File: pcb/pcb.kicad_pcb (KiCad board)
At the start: 2 copper layers, 1 part

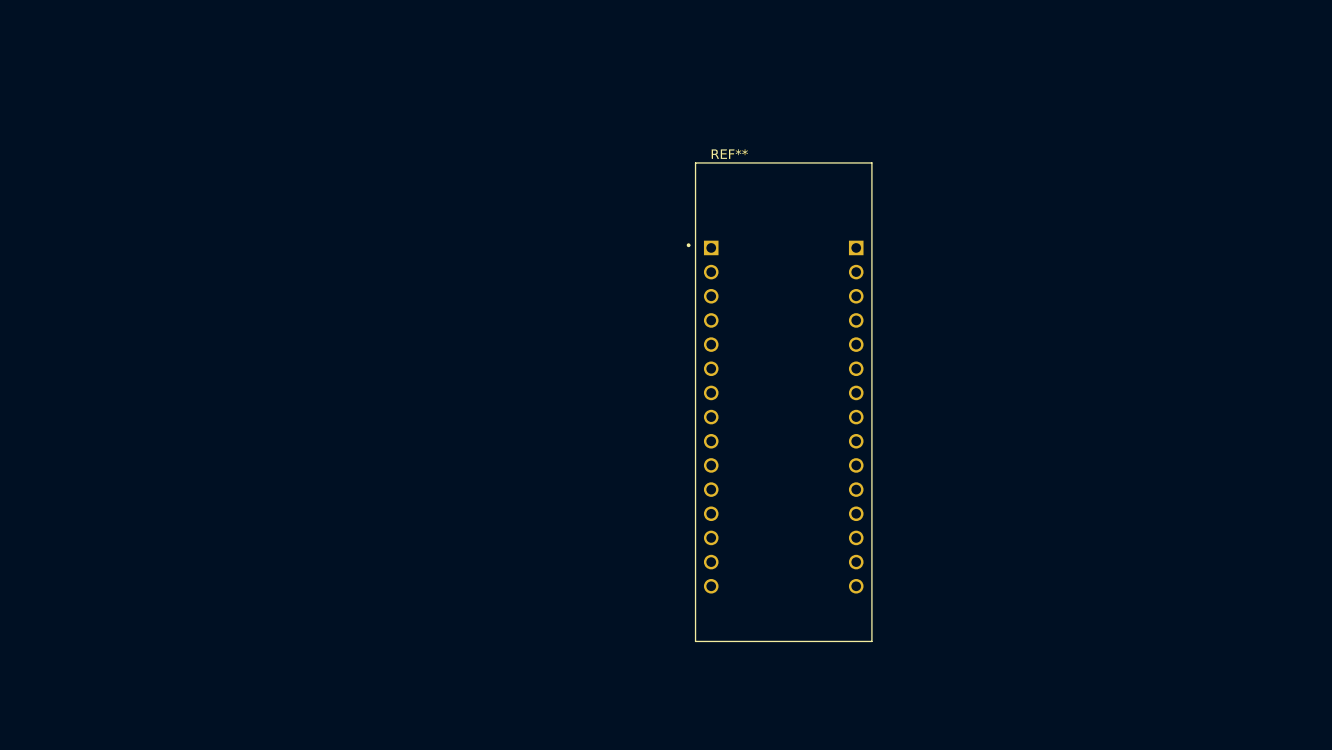
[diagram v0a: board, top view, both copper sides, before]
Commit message: Finalisation PCB
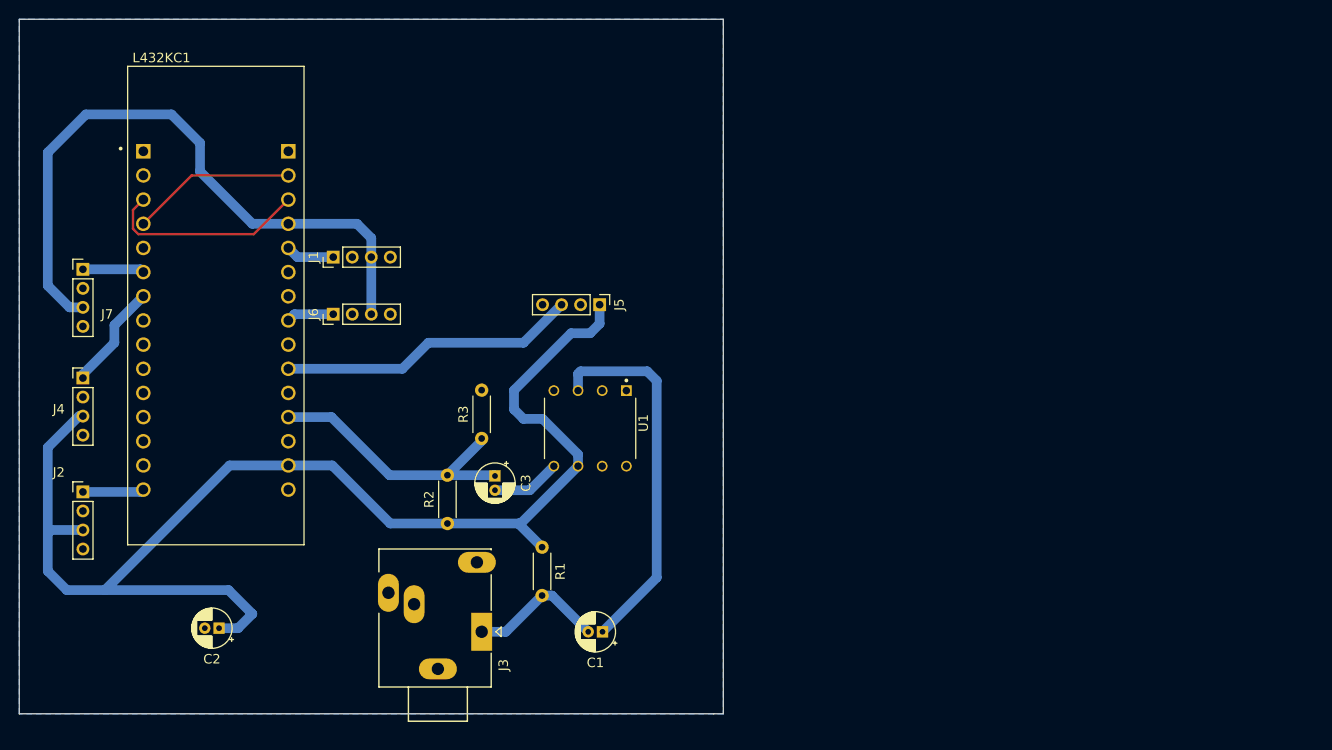
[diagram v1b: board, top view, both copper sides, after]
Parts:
- removed REF**: MODULE_NUCLEO-L432KC, NUCLEO-L432KC:MODULE_NUCLEO-L432KC
- added C1: 1n, Capacitor_THT:CP_Radial_D4.0mm_P1.50mm, F.Cu at (114.3, 119.4)
- added C2: 10u, Capacitor_THT:CP_Radial_D4.0mm_P1.50mm, F.Cu at (74.0, 119.0)
- added C3: 1u, Capacitor_THT:CP_Radial_D4.0mm_P1.50mm, F.Cu at (103.0, 103.0)
- added J1: VIN VBAT, Connector_PinHeader_2.00mm:PinHeader_1x04_P2.00mm_Vertical, F.Cu at (86.0, 80.0)
- added J2: Conn_01x04, Connector_PinHeader_2.00mm:PinHeader_1x04_P2.00mm_Vertical, F.Cu at (59.7, 104.7)
- added J3: AudioJack3, Connector_Audio:Jack_3.5mm_Ledino_KB3SPRS_Horizontal, F.Cu at (101.6, 119.4)
- added J4: Conn_01x04, Connector_PinHeader_2.00mm:PinHeader_1x04_P2.00mm_Vertical, F.Cu at (59.7, 92.7)
- added J5: HX711, Connector_PinHeader_2.00mm:PinHeader_1x04_P2.00mm_Vertical, F.Cu at (114.0, 85.0)
- added J6: Conn_01x04, Connector_PinHeader_2.00mm:PinHeader_1x04_P2.00mm_Vertical, F.Cu at (86.0, 86.0)
- added J7: Conn_01x04, Connector_PinHeader_2.00mm:PinHeader_1x04_P2.00mm_Vertical, F.Cu at (59.7, 81.3)
- added L432KC1: NUCLEO_L432KC, NUCLEO-L432KC:MODULE_NUCLEO-L432KC, F.Cu at (73.7, 85.1)
- added R1: 4.7k, Resistor_THT:R_Axial_DIN0204_L3.6mm_D1.6mm_P5.08mm_Horizontal, F.Cu at (108.0, 110.5)
- added R2: 10k, Resistor_THT:R_Axial_DIN0204_L3.6mm_D1.6mm_P5.08mm_Horizontal, F.Cu at (98.0, 108.0)
- added R3: 10k, Resistor_THT:R_Axial_DIN0204_L3.6mm_D1.6mm_P5.08mm_Horizontal, F.Cu at (101.6, 99.1)
- added U1: LM386, LM386N-4_NOPB:DIP794W45P254L959H508Q8, F.Cu at (113.0, 98.0)
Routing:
- net /+3V3: track 0.00 -> 138.9 mm
- net /+5V: track 0.00 -> 69.4 mm
- net Net-(C1-Pad1): track 0.00 -> 39.3 mm
- net /A2: track 0.00 -> 31.5 mm
- net /A0: track 0.00 -> 29.6 mm
- net Net-(L432KC1-PadNRST): track 0.00 -> 21.6 mm
- net GND: track 0.00 -> 17.3 mm
- net Net-(C1-Pad2): track 0.00 -> 14.4 mm
- net /D4: track 0.00 -> 11.2 mm
- net Net-(C3-Pad2): track 0.00 -> 7.24 mm
- net /D3: track 0.00 -> 6.47 mm
- net /D12: track 0.00 -> 6.45 mm
- net /A7: track 0.00 -> 5.12 mm
- net /A4: track 0.00 -> 4.99 mm
- added copper zone on B.Cu, net GND
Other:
- board outline added: 74 x 73 mm
- board text added: "HX711"

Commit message: Finalisation PCB
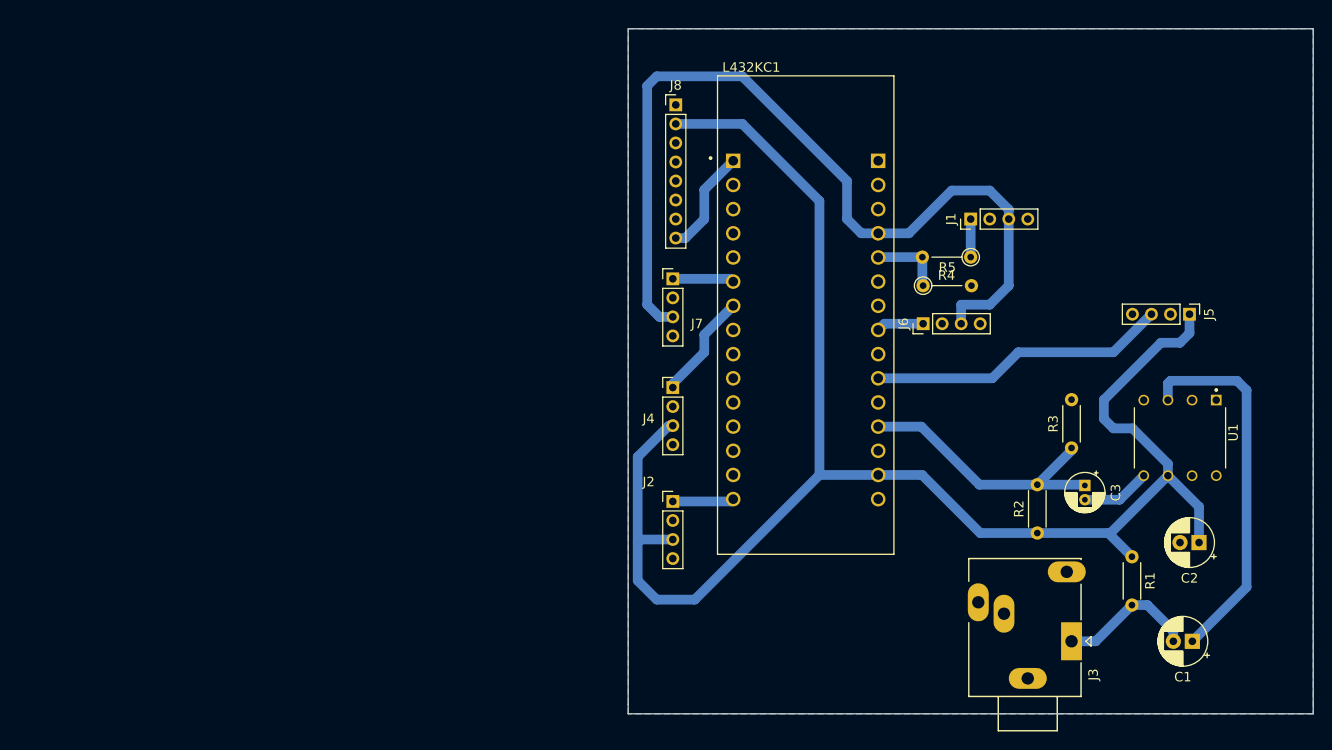
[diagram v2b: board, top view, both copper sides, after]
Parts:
- added J8: Conn_01x08, Connector_PinHeader_2.00mm:PinHeader_1x08_P2.00mm_Vertical, F.Cu at (122.0, 64.0)
- added R4: 2k, Resistor_THT:R_Axial_DIN0204_L3.6mm_D1.6mm_P5.08mm_Vertical, F.Cu at (153.0, 80.0)
- added R5: 1k, Resistor_THT:R_Axial_DIN0204_L3.6mm_D1.6mm_P5.08mm_Vertical, F.Cu at (148.0, 83.0)
- C1: value 1n -> 1u; footprint Capacitor_THT:CP_Radial_D4.0mm_P1.50mm -> Capacitor_THT:CP_Radial_D5.0mm_P2.00mm
- C2: footprint Capacitor_THT:CP_Radial_D4.0mm_P1.50mm -> Capacitor_THT:CP_Radial_D5.0mm_P2.00mm
- moved C2 103.4 mm to (177.0, 110.0)
- moved J1 67.1 mm to (153.0, 76.0)
- moved C1 62.0 mm to (176.3, 120.4)
- moved C3 62.0 mm to (165.0, 104.0)
- moved J2 62.0 mm to (121.7, 105.7)
- moved J3 62.0 mm to (163.6, 120.4)
- moved J4 62.0 mm to (121.7, 93.7)
- moved J5 62.0 mm to (176.0, 86.0)
- moved J6 62.0 mm to (148.0, 87.0)
- moved J7 62.0 mm to (121.7, 82.3)
- moved L432KC1 62.0 mm to (135.7, 86.1)
- moved R2 62.0 mm to (160.0, 109.0)
- moved R3 62.0 mm to (163.6, 100.1)
- moved U1 62.0 mm to (175.0, 99.0)
- moved R1 62.0 mm to (169.9, 111.5)
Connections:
- J1 pad 1: /A7 -> Net-(J1-Pad1)
- J6 pad 2: Net-(J6-Pad2) -> GND
- L432KC1 pad PA9: Net-(L432KC1-PadPA9) -> /D1
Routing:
- net /+3V3: track 138.9 -> 173.9 mm
- net /+5V: track 69.4 -> 92.3 mm
- net Net-(L432KC1-PadNRST): track 21.6 -> 0.00 mm
- net GND: track 17.3 -> 0.00 mm
- net /D1: track 0.00 -> 11.2 mm
- net Net-(J1-Pad1): track 0.00 -> 4.00 mm
- net /A7: track 5.12 -> 7.69 mm
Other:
- board size 74 x 73 mm -> 72 x 72 mm
